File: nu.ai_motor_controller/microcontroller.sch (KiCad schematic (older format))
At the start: 22 parts

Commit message: automated commit
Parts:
- added R?: CR0603-JW-103ELF, 0603, symbol custom:CR0603-JW-103ELF
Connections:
- net labels added: BAT_0, BAT_1, BAT_2, BAT_TESTn, JTAG_TCK, JTAG_TDI, JTAG_TDO, JTAG_TMS, L_DIR, R_DIR
- net labels removed: ADC_0, ADC_1, ADC_11, ADC_4, ADC_5, ADC_6, ADC_7, ADC_8, ADC_9, AIN0, HWBn, PWM_1A, PWM_1B
- wire segments 129 -> 126
- no-connect marks 2 -> 3
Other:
- note added: "ADC_0"
- note added: "ADC_1"
- note added: "ADC_11"
- note added: "ADC_4"
- note added: "ADC_5"
- note added: "ADC_6"
- note added: "ADC_7"
- note added: "ADC_8"
- note added: "ADC_9"
- note added: "PWM_1A"
- note added: "PWM_1B"
- note removed: "GPIO"
- note removed: "L_DIRECTION?\n"
- note removed: "}\n} BAT MONITOR?\n}"
- note removed: "}\n} JTAG/ADC/GPIO\n}\n}"
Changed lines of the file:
@@
 P 4025 3600
 F 0 "U?" H 3525 5350 50  0000 L BNN
-F 1 "ATmega32U4-AU" H 4125 1850 50  0000 L TNN
+F 1 "ATmega32U4-AU" H 4050 1850 50  0000 L TNN
 F 2 "Package_QFP:TQFP-44_10x10mm_P0.8mm" H 4025 3600 50  0001 C CIN
 F 3 "http://ww1.microchip.com/downloads/en/DeviceDoc/Atmel-7766-8-bit-AVR-ATmega16U4-32U4_Datasheet.pdf" H 4025 3600 50  0001 C CNN
@@
 L power:+5V #PWR?
 U 1 1 5C416CFF
-P 3275 1350
-F 0 "#PWR?" H 3275 1200 50  0001 C CNN
-F 1 "+5V" H 3275 1490 50  0000 C CNN
-F 2 "" H 3275 1350 50  0001 C CNN
-F 3 "" H 3275 1350 50  0001 C CNN
-	1    3275 1350
-	1    0    0    -1
-$EndComp
-Wire Wire Line
-	3275 1350 3275 1500
+P 3275 1300
+F 0 "#PWR?" H 3275 1150 50  0001 C CNN
+F 1 "+5V" H 3275 1440 50  0000 C CNN
+F 2 "" H 3275 1300 50  0001 C CNN
+F 3 "" H 3275 1300 50  0001 C CNN
+	1    3275 1300
+	1    0    0    -1
+$EndComp
+Wire Wire Line
+	3275 1300 3275 1500
 $Comp
 L power:GND #PWR?
@@
 	3675 6125 3675 6075
 Wire Wire Line
-	3875 1800 3875 1725
+	3875 1800 3875 1750
 Wire Wire Line
 	4075 1300 4075 1350
@@
 Wire Wire Line
 	2175 1750 1625 1750
-Text Label 5100 2100 2    50   ~ 0
-SPI_SSn
-Text Label 5100 2200 2    50   ~ 0
-SPI_SCK
-Text Label 5100 2300 2    50   ~ 0
-SPI_MOSI
-Text Label 5100 2400 2    50   ~ 0
-SPI_MISO
-Text Label 5100 2500 2    50   ~ 0
-ADC_11
-Text Label 5100 2600 2    50   ~ 0
-PWM_1A
-Text Label 5100 2700 2    50   ~ 0
-PWM_1B
-Text Label 5100 2800 2    50   ~ 0
-PWM_0A
-Wire Wire Line
-	5100 2500 4675 2500
-Text Notes 7325 3425 0    50   ~ 0
-}\n} BAT MONITOR?\n}
-Text Label 5100 3100 2    50   ~ 0
-PWM_4A
-Text Label 5100 3000 2    50   ~ 0
-PWM_3A
-Text Label 5100 3300 2    50   ~ 0
-I2C_SCL
-Text Label 5100 3400 2    50   ~ 0
-I2C_SDA
-Text Label 5100 3500 2    50   ~ 0
-USART_RX
-Text Label 5100 3600 2    50   ~ 0
-USART_TX
-Text Label 5100 3700 2    50   ~ 0
-ADC_8
-Text Label 5100 3900 2    50   ~ 0
-ADC_9
-Text Label 5100 4300 2    50   ~ 0
-AIN0
-Text Label 5100 4200 2    50   ~ 0
-HWBn
-Text Label 5100 4500 2    50   ~ 0
-ADC_0
-Text Label 5100 4600 2    50   ~ 0
-ADC_1
-Text Label 5100 4700 2    50   ~ 0
-ADC_4
-Text Label 5100 4800 2    50   ~ 0
-ADC_5
-Text Label 5100 4900 2    50   ~ 0
-ADC_6
-Text Label 5100 5000 2    50   ~ 0
-ADC_7
-Wire Wire Line
-	4675 4700 5400 4700
-Wire Wire Line
-	4675 4800 5400 4800
-Wire Wire Line
-	4675 4900 5400 4900
-Wire Wire Line
-	4675 5000 5400 5000
-Text Notes 5475 5000 0    50   ~ 0
-}\n} JTAG/ADC/GPIO\n}\n}
-Text Notes 5100 3800 2    50   ~ 0
-GPIO
-Text Label 5100 4000 2    50   ~ 0
-PWM_4D
-Wire Wire Line
-	4675 2600 6000 2600
-Wire Wire Line
-	4675 2700 6000 2700
-Text HLabel 6000 2600 2    50   Input ~ 0
-MOTOR_L
-Text HLabel 6000 2700 2    50   Input ~ 0
-MOTOR_R
-Wire Wire Line
-	5400 2800 5400 2900
-Wire Wire Line
-	5400 2900 5750 2900
-Wire Wire Line
-	4675 2800 5400 2800
-Wire Wire Line
-	4675 3000 5750 3000
-Wire Wire Line
-	4675 3100 5750 3100
-Wire Wire Line
-	5400 4000 5400 3200
-Wire Wire Line
-	5400 3200 5750 3200
-Wire Wire Line
-	4675 4000 5400 4000
-Wire Wire Line
-	4675 2100 5750 2100
-Wire Wire Line
-	4675 2200 5750 2200
-Wire Wire Line
-	4675 2300 5750 2300
-Wire Wire Line
-	4675 2400 5750 2400
-Wire Wire Line
-	4675 4500 5200 4500
-Wire Wire Line
-	5200 4500 5200 4400
-Wire Wire Line
-	5200 4400 5400 4400
-Wire Wire Line
-	5300 4600 5300 4500
-Wire Wire Line
-	5300 4500 5400 4500
-Wire Wire Line
-	4675 4600 5300 4600
-Wire Wire Line
-	4675 3300 6000 3300
-Wire Wire Line
-	6000 3400 4675 3400
-Wire Wire Line
-	4675 3500 5750 3500
-Wire Wire Line
-	5750 3600 4675 3600
-Wire Wire Line
-	4675 3800 6000 3800
+Wire Wire Line
+	5200 2500 4675 2500
+Wire Wire Line
+	4675 4700 5200 4700
+Wire Wire Line
+	4675 4800 5200 4800
+Wire Wire Line
+	4675 4900 5200 4900
+Wire Wire Line
+	4675 5000 5200 5000
+Wire Wire Line
+	4675 2600 5200 2600
+Wire Wire Line
+	4675 2700 5200 2700
+Wire Wire Line
+	4675 3000 5200 3000
+Wire Wire Line
+	4675 3100 5200 3100
+Wire Wire Line
+	4675 2100 5200 2100
+Wire Wire Line
+	4675 2200 5200 2200
+Wire Wire Line
+	4675 2300 5200 2300
+Wire Wire Line
+	4675 2400 5200 2400
+Wire Wire Line
+	4675 3300 5200 3300
+Wire Wire Line
+	5200 3400 4675 3400
+Wire Wire Line
+	4675 3500 5200 3500
+Wire Wire Line
+	5200 3600 4675 3600
+Wire Wire Line
+	4675 3800 5200 3800
 Wire Wire Line
 	4275 1750 4175 1750
@@
 	4075 1350 4175 1350
 Wire Wire Line
-	4075 1725 3975 1725
-Wire Wire Line
-	4075 1725 4075 1800
-Connection ~ 3975 1725
-Wire Wire Line
-	3975 1725 3975 1800
+	4075 1750 3975 1750
+Wire Wire Line
+	4075 1750 4075 1800
+Connection ~ 3975 1750
+Wire Wire Line
+	3975 1750 3975 1800
 Wire Wire Line
 	4175 1750 4175 1800
@@
 	3775 5500 3675 5500
 Wire Wire Line
-	3975 1725 3875 1725
-Wire Wire Line
-	4075 1350 4075 1725
+	3975 1750 3875 1750
+Wire Wire Line
+	4075 1350 4075 1750
 Connection ~ 4075 1350
-Connection ~ 4075 1725
-Text Notes 6000 3800 2    50   ~ 0
-L_DIRECTION?\n
-Text HLabel 5750 2100 2    50   Input ~ 0
+Connection ~ 4075 1750
+Wire Wire Line
+	4675 3700 5200 3700
+Wire Wire Line
+	4675 3900 5200 3900
+Wire Wire Line
+	4675 4500 5200 4500
+Wire Wire Line
+	4675 4600 5200 4600
+Wire Wire Line
+	4675 2800 5200 2800
+Wire Wire Line
+	4675 4000 5200 4000
+Text Notes 5100 2500 2    50   ~ 0
+ADC_11
+Text Notes 5100 2600 2    50   ~ 0
+PWM_1A
+Text Notes 5100 2700 2    50   ~ 0
+PWM_1B
+Text Notes 5100 3700 2    50   ~ 0
+ADC_8
+Text Notes 5100 3900 2    50   ~ 0
+ADC_9
+Text Notes 5100 4500 2    50   ~ 0
+ADC_0
+NoConn ~ 4675 4300
+Wire Wire Line
+	5425 4200 5200 4200
+Wire Wire Line
+	5425 4250 5425 4200
+$Comp
+L power:GND #PWR?
+U 1 1 5C4CEC30
+P 5425 4250
+F 0 "#PWR?" H 5425 4000 50  0001 C CNN
+F 1 "GND" H 5425 4100 50  0000 C CNN
+F 2 "" H 5425 4250 50  0001 C CNN
+F 3 "" H 5425 4250 50  0001 C CNN
+	1    5425 4250
+	1    0    0    -1
+$EndComp
+$Comp
+L custom:CR0603-JW-103ELF R?
+U 1 1 5C4CE88E
+P 5050 4200
+F 0 "R?" V 4990 4160 50  0000 L BNN
+F 1 "CR0603-JW-103ELF" V 5175 3875 50  0001 L BNN
+F 2 "0603" V 5250 4100 50  0001 L BNN
+F 3 "~/datasheets/chpreztr.pdf" V 5350 3750 50  0001 L BNN
+F 4 "10k" V 5080 4130 50  0000 L BNN "Resistance"
+	1    5050 4200
+	0    1    1    0
+$EndComp
+Wire Wire Line
+	4675 4200 4900 4200
+Text Notes 5100 4600 2    50   ~ 0
+ADC_1
+Text GLabel 5200 2100 2    50   Input ~ 0
 SPI_SSn
-Text HLabel 5750 2200 2    50   Input ~ 0
+Text GLabel 5200 2200 2    50   Input ~ 0
 SPI_SCK
-Text HLabel 5750 2300 2    50   Input ~ 0
+Text GLabel 5200 2300 2    50   Input ~ 0
 SPI_MOSI
-Text HLabel 5750 2400 2    50   Input ~ 0
+Text GLabel 5200 2400 2    50   Input ~ 0
 SPI_MISO
-Text HLabel 5750 2900 2    50   Input ~ 0
+Text GLabel 5200 2500 2    50   Input ~ 0
+BAT_2
+Text GLabel 5200 2600 2    50   Input ~ 0
+MOTOR_L
+Text GLabel 5200 2700 2    50   Input ~ 0
+MOTOR_R
+Text GLabel 5200 2800 2    50   Input ~ 0
 PWM_0A
-Text HLabel 5750 3000 2    50   Input ~ 0
+Text GLabel 5200 3000 2    50   Input ~ 0
 PWM_3A
-Text HLabel 5750 3100 2    50   Input ~ 0
+Text GLabel 5200 3100 2    50   Input ~ 0
 PWM_4A
-Text HLabel 5750 3200 2    50   Input ~ 0
+Text GLabel 5200 3300 2    50   Input ~ 0
+I2C_SCL
+Text GLabel 5200 3400 2    50   Input ~ 0
+I2C_SDA
+Text GLabel 5200 3500 2    50   Input ~ 0
+USART_RX
+Text GLabel 5200 3600 2    50   Input ~ 0
+USART_TX
+Text GLabel 5200 3700 2    50   Input ~ 0
+BAT_0
+Text GLabel 5200 3800 2    50   Input ~ 0
+L_DIR
+Text GLabel 5200 3900 2    50   Input ~ 0
+BAT_1
+Text GLabel 5200 4000 2    50   Input ~ 0
 PWM_4D
-Text HLabel 6000 3300 2    50   Input ~ 0
-I2C_SCL
-Text HLabel 6000 3400 2    50   Input ~ 0
-I2C_SDA
-Text HLabel 5750 3500 2    50   Input ~ 0
-USART_RX
-Text HLabel 5750 3600 2    50   Input ~ 0
-USART_TX
+Text GLabel 5200 4500 2    50   Input ~ 0
+R_DIR
+Text GLabel 5200 4600 2    50   Input ~ 0
+BAT_TESTn
+Text GLabel 5200 4700 2    50   Input ~ 0
+JTAG_TDI
+Text GLabel 5200 4800 2    50   Input ~ 0
+JTAG_TDO
+Text GLabel 5200 4900 2    50   Input ~ 0
+JTAG_TMS
+Text GLabel 5200 5000 2    50   Input ~ 0
+JTAG_TCK
+Text Notes 5100 4700 2    50   ~ 0
+ADC_4
+Text Notes 5100 4800 2    50   ~ 0
+ADC_5
+Text Notes 5100 4900 2    50   ~ 0
+ADC_6
+Text Notes 5100 5000 2    50   ~ 0
+ADC_7
 $EndSCHEMATC

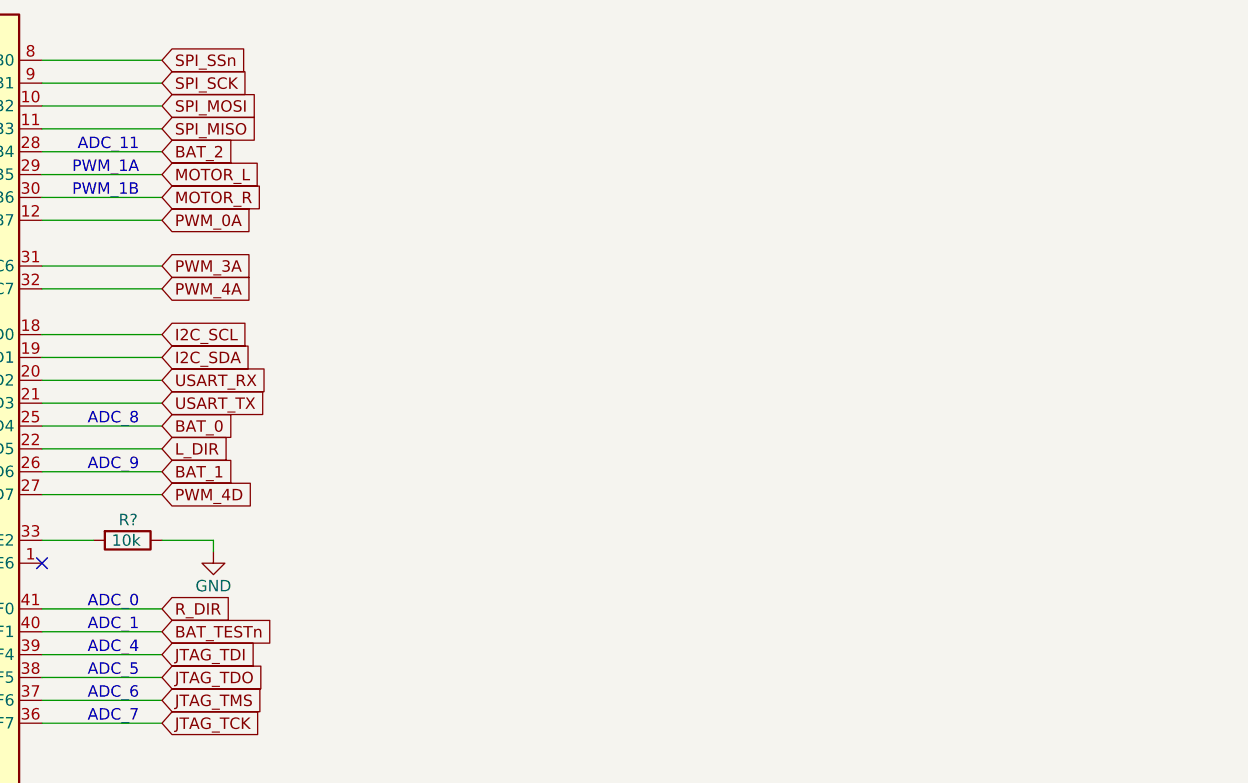
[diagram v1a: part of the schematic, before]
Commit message: automated commit
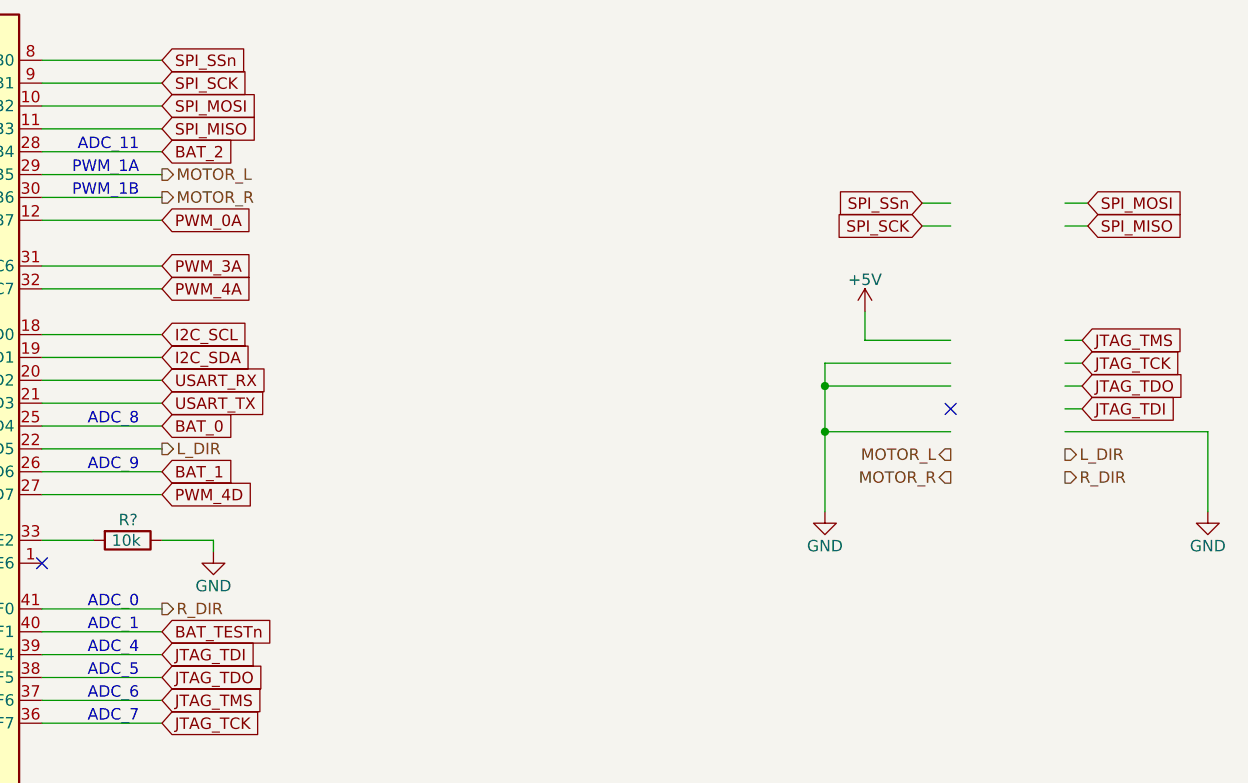
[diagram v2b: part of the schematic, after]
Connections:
- wire segments 126 -> 144
- no-connect marks 3 -> 4
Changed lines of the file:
@@
 Text GLabel 5200 2500 2    50   Input ~ 0
 BAT_2
-Text GLabel 5200 2600 2    50   Input ~ 0
-MOTOR_L
-Text GLabel 5200 2700 2    50   Input ~ 0
-MOTOR_R
 Text GLabel 5200 2800 2    50   Input ~ 0
 PWM_0A
@@
 Text GLabel 5200 3700 2    50   Input ~ 0
 BAT_0
-Text GLabel 5200 3800 2    50   Input ~ 0
-L_DIR
 Text GLabel 5200 3900 2    50   Input ~ 0
 BAT_1
 Text GLabel 5200 4000 2    50   Input ~ 0
 PWM_4D
-Text GLabel 5200 4500 2    50   Input ~ 0
-R_DIR
 Text GLabel 5200 4600 2    50   Input ~ 0
 BAT_TESTn
@@
 Text Notes 5100 5000 2    50   ~ 0
 ADC_7
+Text GLabel 8525 2725 0    50   Input ~ 0
+SPI_SSn
+Text GLabel 8525 2825 0    50   Input ~ 0
+SPI_SCK
+Text GLabel 9250 2725 2    50   Input ~ 0
+SPI_MOSI
+Text GLabel 9250 2825 2    50   Input ~ 0
+SPI_MISO
+Wire Wire Line
+	9250 2825 9150 2825
+Wire Wire Line
+	9150 2725 9250 2725
+Wire Wire Line
+	8525 2725 8650 2725
+Wire Wire Line
+	8650 2825 8525 2825
+Text GLabel 9225 3325 2    50   Input ~ 0
+JTAG_TMS
+Text GLabel 9225 3425 2    50   Input ~ 0
+JTAG_TCK
+Text GLabel 9225 3525 2    50   Input ~ 0
+JTAG_TDO
+Text GLabel 9225 3625 2    50   Input ~ 0
+JTAG_TDI
+$Comp
+L power:GND #PWR?
+U 1 1 5C4A6E4A
+P 8100 4075
+F 0 "#PWR?" H 8100 3825 50  0001 C CNN
+F 1 "GND" H 8100 3925 50  0000 C CNN
+F 2 "" H 8100 4075 50  0001 C CNN
+F 3 "" H 8100 4075 50  0001 C CNN
+	1    8100 4075
+	1    0    0    -1
+$EndComp
+Wire Wire Line
+	8100 3425 8650 3425
+Wire Wire Line
+	8650 3525 8100 3525
+Wire Wire Line
+	8100 3425 8100 3525
+Connection ~ 8100 3525
+Wire Wire Line
+	8100 3525 8100 3725
+$Comp
+L power:+5V #PWR?
+U 1 1 5C4B092D
+P 8275 3200
+F 0 "#PWR?" H 8275 3050 50  0001 C CNN
+F 1 "+5V" H 8275 3340 50  0000 C CNN
+F 2 "" H 8275 3200 50  0001 C CNN
+F 3 "" H 8275 3200 50  0001 C CNN
+	1    8275 3200
+	1    0    0    -1
+$EndComp
+Wire Wire Line
+	8275 3200 8275 3325
+Wire Wire Line
+	8275 3325 8650 3325
+NoConn ~ 8650 3625
+Wire Wire Line
+	9225 3325 9150 3325
+Wire Wire Line
+	9225 3425 9150 3425
+Wire Wire Line
+	9225 3525 9150 3525
+Wire Wire Line
+	9225 3625 9150 3625
+Text HLabel 8650 3825 0    50   Output ~ 0
+MOTOR_L
+Text HLabel 8650 3925 0    50   Output ~ 0
+MOTOR_R
+Text HLabel 5200 2600 2    50   Output ~ 0
+MOTOR_L
+Text HLabel 5200 2700 2    50   Output ~ 0
+MOTOR_R
+Text HLabel 9150 3825 2    50   Output ~ 0
+L_DIR
+Text HLabel 9150 3925 2    50   Output ~ 0
+R_DIR
+Text HLabel 5200 3800 2    50   Output ~ 0
+L_DIR
+Text HLabel 5200 4500 2    50   Output ~ 0
+R_DIR
+Wire Wire Line
+	8650 3725 8100 3725
+Connection ~ 8100 3725
+Wire Wire Line
+	8100 3725 8100 4075
+$Comp
+L power:GND #PWR?
+U 1 1 5C536053
+P 9775 4075
+F 0 "#PWR?" H 9775 3825 50  0001 C CNN
+F 1 "GND" H 9775 3925 50  0000 C CNN
+F 2 "" H 9775 4075 50  0001 C CNN
+F 3 "" H 9775 4075 50  0001 C CNN
+	1    9775 4075
+	1    0    0    -1
+$EndComp
+Wire Wire Line
+	9775 3725 9775 4075
+Wire Wire Line
+	9775 3725 9150 3725
 $EndSCHEMATC

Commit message: automated commit
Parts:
- removed C?: NP_C_0603, Capacitor_SMD:C_0603_1608Metric, symbol custom:NP_C_0603
- removed C?: NP_C_0402, Capacitor_SMD:C_0402_1005Metric, symbol custom:NP_C_0402
- added C? (x2): CL10B105KA8NNNC, Capacitor_SMD:C_0603_1608Metric, symbol custom:CL10B105KA8NNNC
- added C? (x4): CL10B104KO8NNNC, Capacitor_SMD:C_0603_1608Metric, symbol custom:CL10B104KO8NNNC
- added D?: CM1293A-04SO, SOT-457, symbol custom:CM1293A-04SO
- added J?: Conn_02x05_Odd_Even, symbol Connector_Generic:Conn_02x05_Odd_Even
- added J?: Conn_02x12_Odd_Even, symbol Connector_Generic:Conn_02x12_Odd_Even
- added SW?: TACTILE_SWITCH, symbol custom:TACTILE_SWITCH
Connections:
- net labels added: +3V3, RESET
- wire segments 144 -> 204
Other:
- note added: "PLACE CLOSE TO\nTACTILE SWITCH"
- moved on the sheet: C?, D?, F?, J?, L?, R?, U?, Y?
